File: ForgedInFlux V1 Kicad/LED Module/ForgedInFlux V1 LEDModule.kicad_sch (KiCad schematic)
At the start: 30 parts

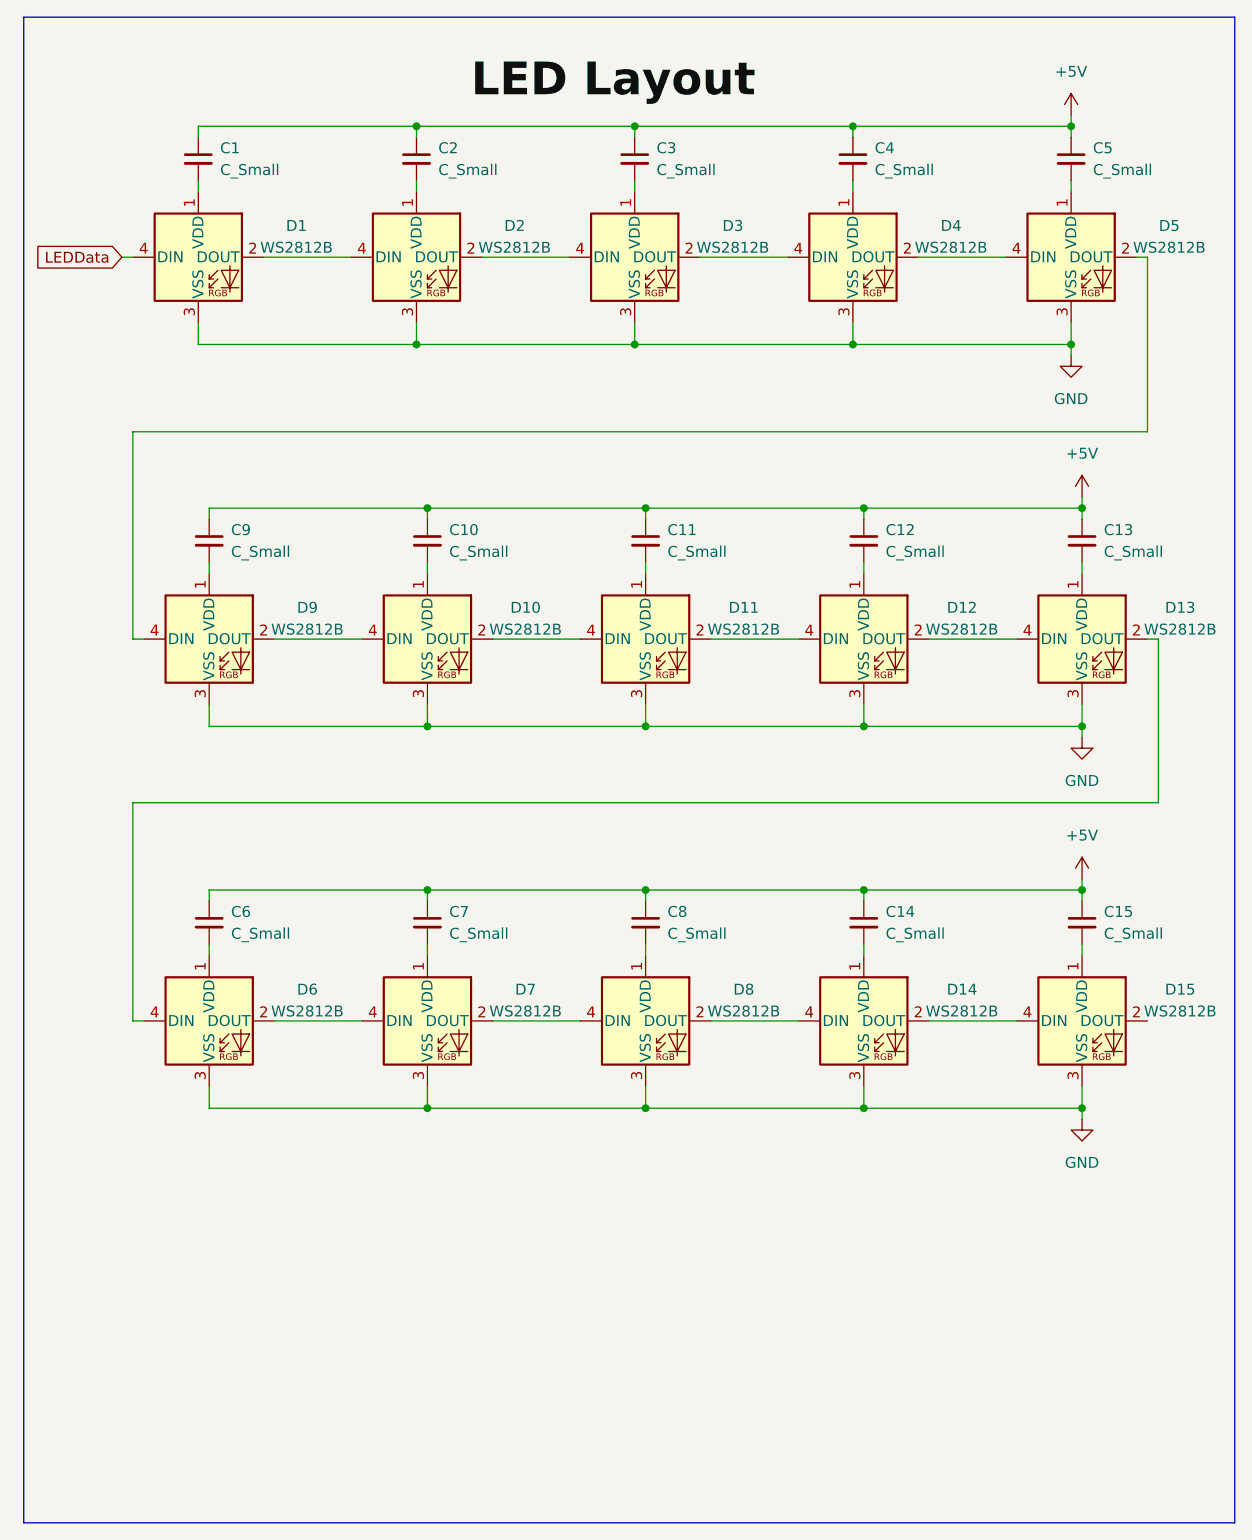
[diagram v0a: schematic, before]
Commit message: Edited Schematic
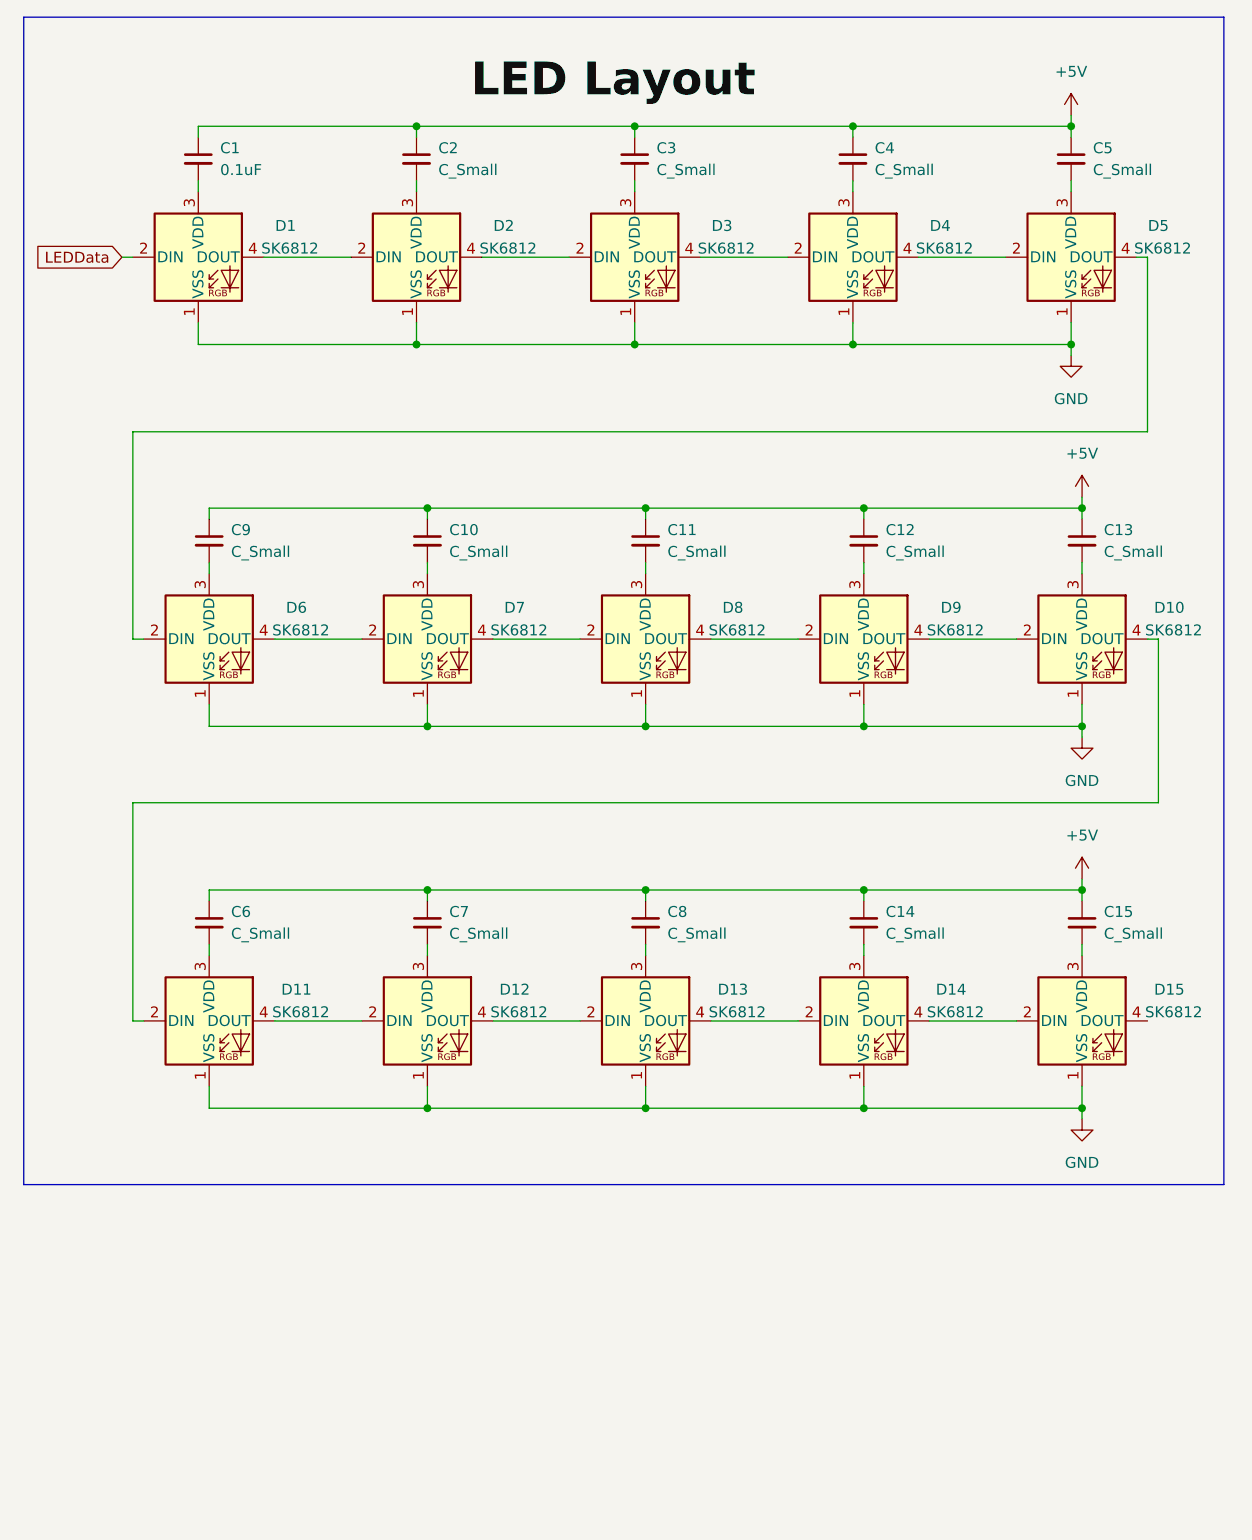
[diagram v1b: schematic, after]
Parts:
- removed D1, D10, D11, D12, D13, D14, D15, D2, D3, D4, D5, D6, D7, D8, D9: WS2812B, LED_SMD:LED_WS2812B_PLCC4_5.0x5.0mm_P3.2mm, symbol LED:WS2812B
- added D1, D10, D11, D12, D13, D14, D15, D2, D3, D4, D5, D6, D7, D8, D9: SK6812, LED_SMD:LED_SK6812_PLCC4_5.0x5.0mm_P3.2mm, symbol LED:SK6812
- C1: value C_Small -> 0.1uF
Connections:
- net GND: now also D1.1 (VSS), D10.1 (VSS), D11.1 (VSS), D12.1 (VSS), D13.1 (VSS), D14.1 (VSS), D15.1 (VSS), D2.1 (VSS), D3.1 (VSS), D4.1 (VSS), D5.1 (VSS), D6.1 (VSS), D7.1 (VSS), D8.1 (VSS), D9.1 (VSS)
- net LEDData: now also D1.2 (DIN)
- net at C9.2: now also D6.3 (VDD)
- net at C8.2: now also D13.3 (VDD)
- net at C14.2: now also D14.3 (VDD)
- net at C15.2: now also D15.3 (VDD)
- net at C11.2: now also D8.3 (VDD)
- net at C4.2: now also D4.3 (VDD)
- net at C2.2: now also D2.3 (VDD)
- net at C12.2: now also D9.3 (VDD)
- net at C1.2: now also D1.3 (VDD)
- net at C6.2: now also D11.3 (VDD)
- net at C13.2: now also D10.3 (VDD)
- net at C5.2: now also D5.3 (VDD)
- net at C10.2: now also D7.3 (VDD)
- net at C3.2: now also D3.3 (VDD)
- net at C7.2: now also D12.3 (VDD)
- new net: D10.4 (DOUT), D11.2 (DIN)
- new net: D11.4 (DOUT), D12.2 (DIN)
- new net: D12.4 (DOUT), D13.2 (DIN)
- new net: D5.4 (DOUT), D6.2 (DIN)
- new net: D6.4 (DOUT), D7.2 (DIN)
- new net: D14.4 (DOUT), D15.2 (DIN)
- new net: D7.4 (DOUT), D8.2 (DIN)
- new net: D2.4 (DOUT), D3.2 (DIN)
- new net: D3.4 (DOUT), D4.2 (DIN)
- new net: D13.4 (DOUT), D14.2 (DIN)
- new net: D1.4 (DOUT), D2.2 (DIN)
- new net: D8.4 (DOUT), D9.2 (DIN)
- new net: D10.2 (DIN), D9.4 (DOUT)
- new net: D4.4 (DOUT), D5.2 (DIN)
